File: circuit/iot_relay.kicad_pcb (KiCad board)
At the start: 2 copper layers, 48.9 x 58.2 mm, 21 parts, among them K1 DIPxx-1Cxx-51x, T1 Transformer_SP_2S, U1 ESP-12F, U2 4N35, U3 AMS1117-3.3

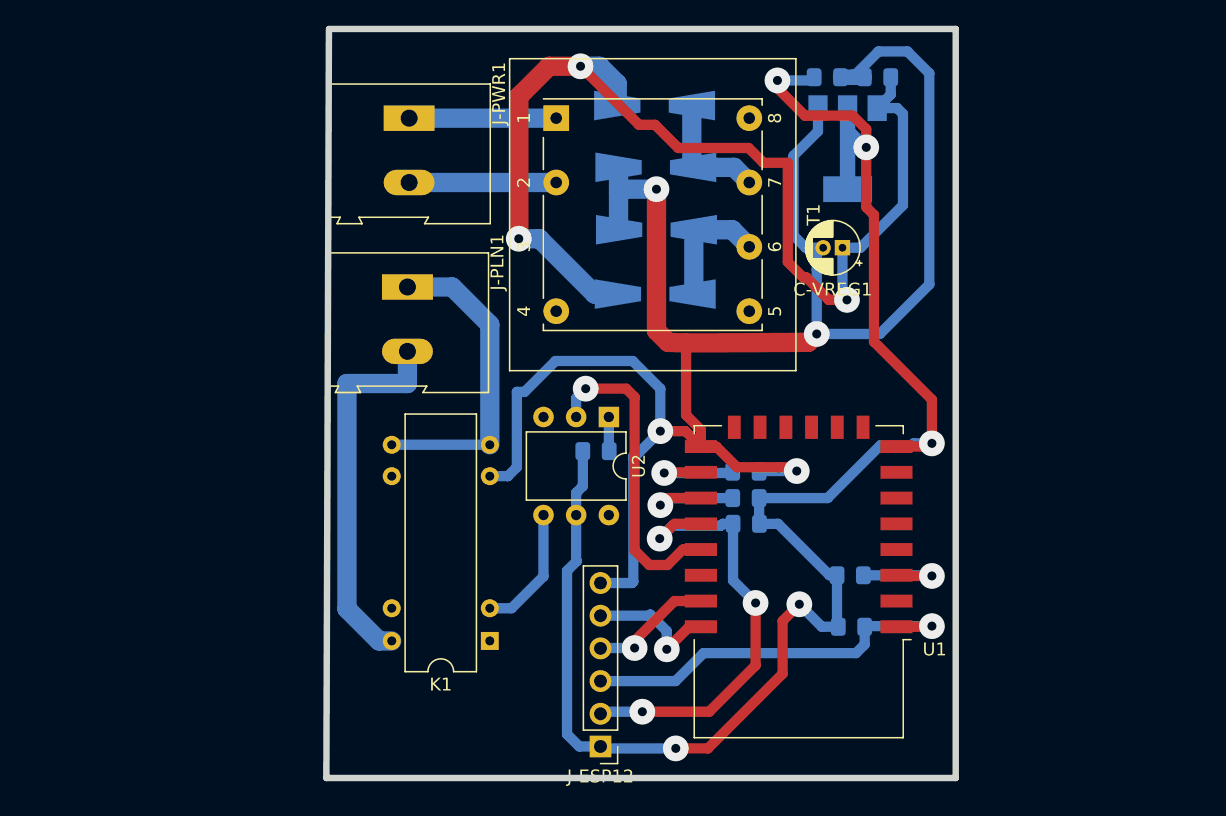
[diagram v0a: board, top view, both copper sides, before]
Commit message: update
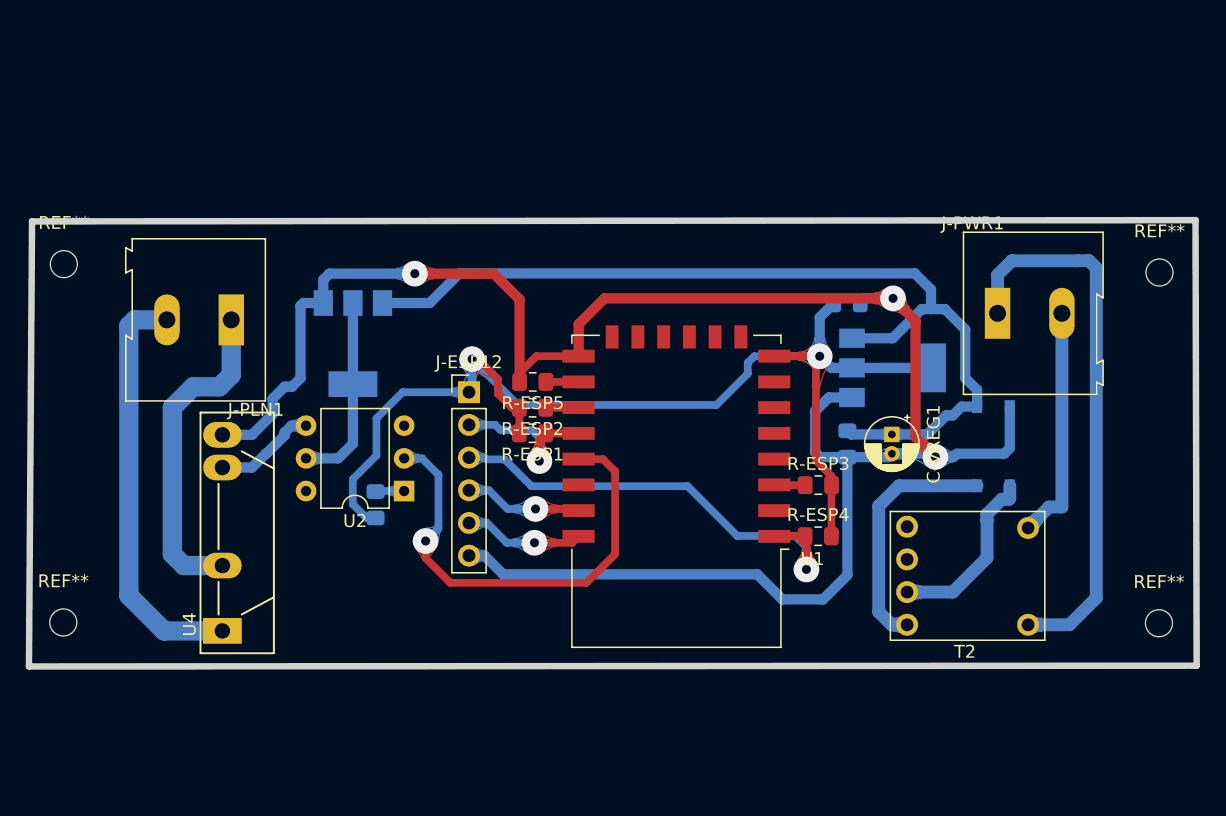
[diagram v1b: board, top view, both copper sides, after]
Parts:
- removed D-VREG1, D-VREG2, D-VREG3, D-VREG4: D, Diode_SMD:D_SMA-SMB_Universal_Handsoldering
- removed K1: DIPxx-1Cxx-51x, Relay_THT:Relay_StandexMeder_DIP_LowProfile
- removed T1: Transformer_SP_2S, Transformer_THT:Transformer_Breve_TEZ-22x24
- added D1: MB6S, Package_TO_SOT_SMD:TO-269AA, B.Cu at (127.1, 58.9)
- added REF**: MountingHole_2.1mm, MountingHole:MountingHole_2.1mm, F.Cu at (54.9, 44.7)
- added REF**: MountingHole_2.1mm, MountingHole:MountingHole_2.1mm, F.Cu at (54.8, 72.6)
- added REF**: MountingHole_2.1mm, MountingHole:MountingHole_2.1mm, F.Cu at (140.0, 72.6)
- added REF**: MountingHole_2.1mm, MountingHole:MountingHole_2.1mm, F.Cu at (140.0, 45.4)
- added T2: Transformer_1P_2S, trafokecil:charger_transformator_a, F.Cu at (124.9, 72.0)
- added U4: S216S01, Package_SIP:SIP4_Sharp-SSR_P7.62mm_Straight, F.Cu at (67.2, 73.2)
- added U5: AMS1117-5.0, Package_TO_SOT_SMD:SOT-223-3_TabPin2, B.Cu at (77.3, 50.9)
- R-ESP1, R-ESP2, R-ESP3, R-ESP4, R-ESP5: moved to F.Cu
- moved J-PWR1 48.2 mm to (127.4, 48.5), turned to 0 degrees
- moved J-ESP12 29.4 mm to (86.3, 54.7), turned to 0 degrees
- moved C-VREG2 28.6 mm to (115.8, 58.7), turned to 270 degrees
- moved R-ESP1 18.0 mm to (91.3, 57.9), turned to 180 degrees
- moved R-ESP2 18.0 mm to (91.3, 55.9), turned to 180 degrees
- moved R-ESP5 18.0 mm to (91.3, 53.9), turned to 180 degrees
- moved C-VREG3 17.6 mm to (115.7, 47.8)
- moved R-OPTO1 17.6 mm to (79.1, 63.4), turned to 90 degrees
- moved U3 17.4 mm to (119.3, 52.8), turned to 0 degrees
- moved U2 16.9 mm to (81.3, 62.4), turned to 180 degrees
- moved C-VREG1 15.0 mm to (119.2, 58.0), turned to 270 degrees
- moved J-PLN1 13.9 mm to (67.9, 49.1), turned to 180 degrees
- moved U1 11.8 mm to (102.5, 62.4)
- moved R-ESP4 7.50 mm to (113.5, 65.9), turned to 0 degrees
- moved R-ESP3 7.43 mm to (113.5, 61.9), turned to 0 degrees
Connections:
- net /V-PWR renamed Net-(C-VREG1-Pad1)
- U2 pad 5: VDD -> VCC
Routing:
- net VDD: track 131.8 -> 89.9 mm, vias 5 -> 2
- net Net-(J-PWR1-Pad1): track 11.4 -> 43.1 mm
- net /P0: track 35.2 -> 12.7 mm, vias 3 -> 1
- net Net-(D1-Pad2): track 0.00 -> 19.1 mm
- net VCC: track 0.00 -> 15.0 mm
- net Net-(D1-Pad1): track 0.00 -> 14.0 mm
- net Net-(C-VREG1-Pad1): track 86.5 -> 73.5 mm, vias 3 -> 0
- net /P_RELAY: track 24.6 -> 36.2 mm
- net /AC1: track 9.90 -> 0.00 mm
- net /AC0: track 9.69 -> 0.00 mm
- net Net-(J-PWR1-Pad2): track 11.4 -> 18.4 mm
- net /P2: track 9.23 -> 2.56 mm, vias 1 -> 0
- net /EN: track 8.12 -> 2.41 mm, vias 1 -> 0
- net /P15: track 8.24 -> 2.54 mm, vias 1 -> 0
- net GND: track 151.8 -> 156.8 mm, vias 4 -> 3
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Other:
- board size 48.9 x 58.2 mm -> 90.7 x 34.7 mm
